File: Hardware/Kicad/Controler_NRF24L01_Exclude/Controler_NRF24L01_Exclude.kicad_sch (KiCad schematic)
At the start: 51 parts, among them J1 Conn_01x02, SW1 SW_Push, SW10 SW_Push, SW11 SW_DIP_x01, SW12 SW_Push, SW13 SW_DIP_x01, SW2 SW_Push, SW3 SW_Push, SW4 SW_Push, SW5 SW_Push, SW6 SW_Push, SW7 SW_Push, SW8 SW_Push, SW9 SW_Push, U1 STM32L412KBTx, U2 MIC5219-3.3YMM, U2 nRF24_Full

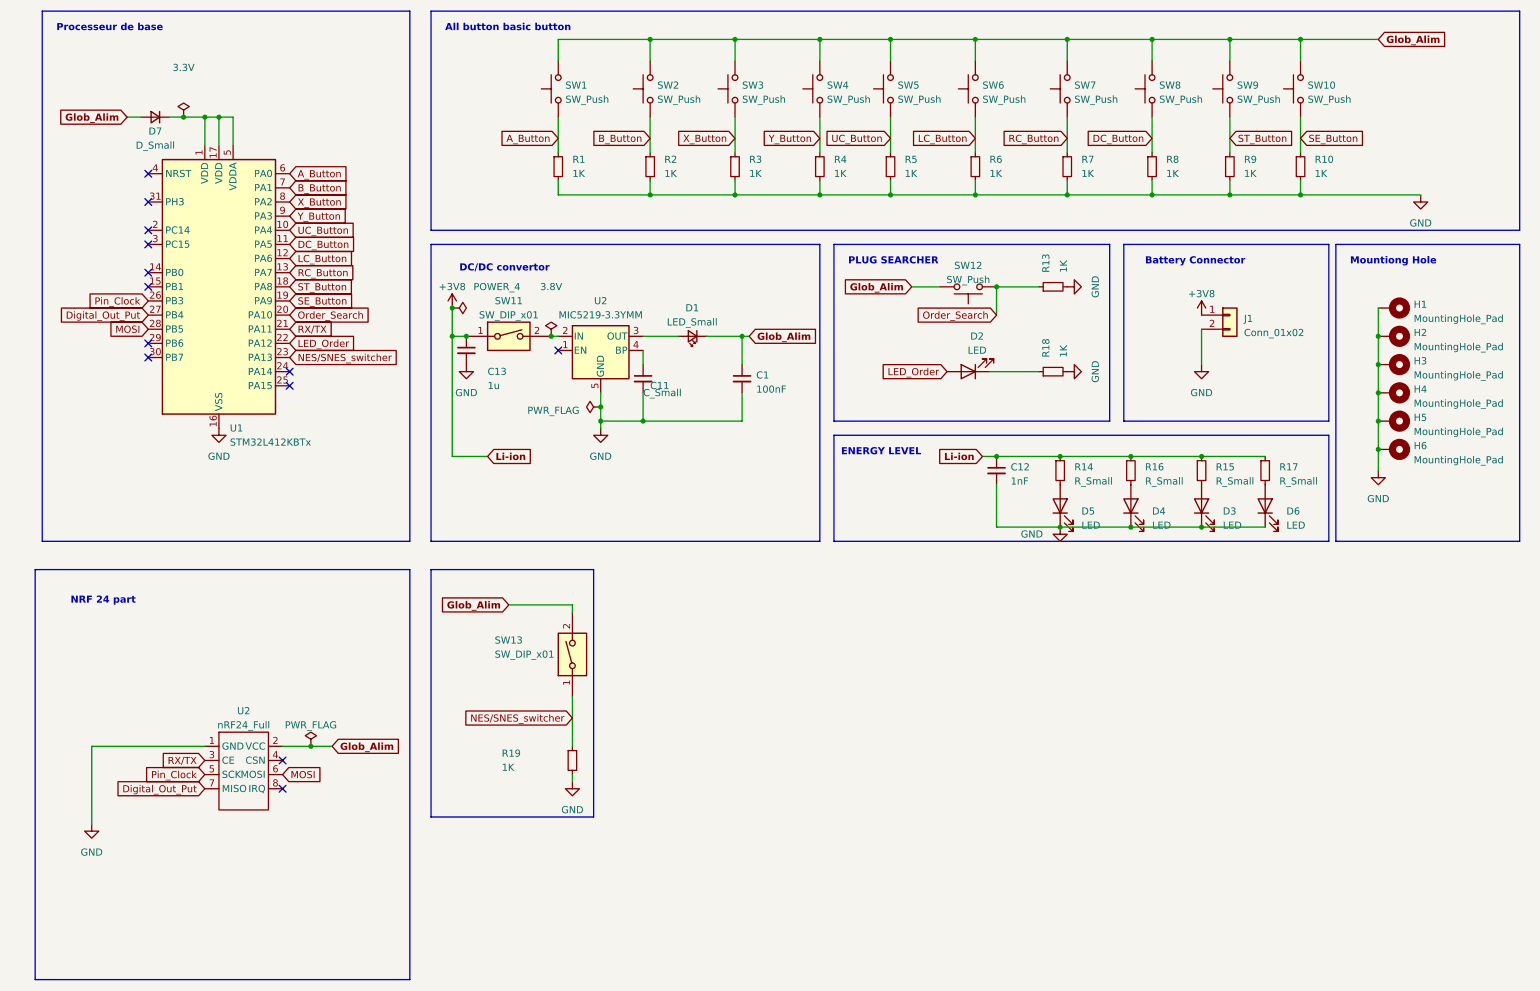
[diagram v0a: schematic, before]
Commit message: correction
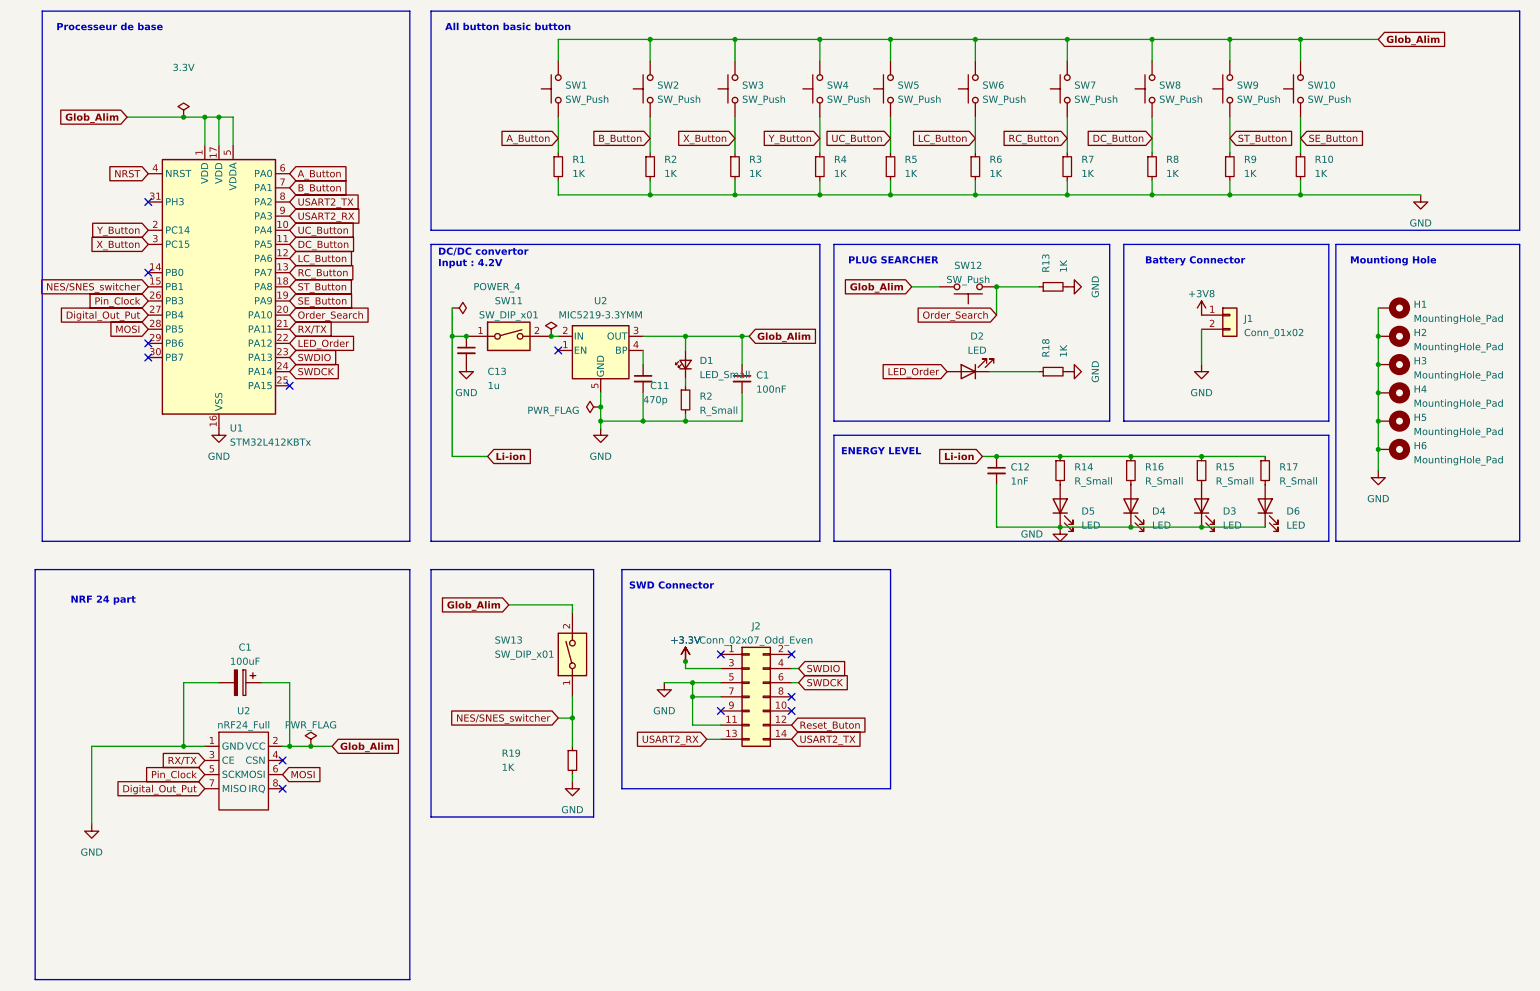
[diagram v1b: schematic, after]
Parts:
- removed D7: D_Small, Diode_SMD:D_0603_1608Metric_Pad1.05x0.95mm_HandSolder, symbol Device:D_Small
- added C1: 100uF, symbol Device:C_Polarized
- added J2: Conn_02x07_Odd_Even, Connector_PinHeader_1.27mm:PinHeader_2x07_P1.27mm_Vertical_SMD, symbol Connector_Generic:Conn_02x07_Odd_Even
- added R2: R_Small, symbol Device:R_Small
- C11: value C_Small -> 470p
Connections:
- net +3V8: no longer C12.1, C13.1, R14.1, R15.1, R16.1, R17.1, SW11.1
- net GND: now also C1.2, J2.11 (Pin_11), J2.5 (Pin_5), J2.7 (Pin_7), R2.2
- net Glob_Alim: now also D1.2 (A), U1.1 (VDD), U1.17 (VDD), U1.5 (VDDA), U2.3 (OUT), C1.1; no longer D1.1 (K)
- net NES/SNES_switcher: now also U1.15 (PB1); no longer U1.23 (PA13)
- net X_Button: now also U1.3 (PC15); no longer U1.8 (PA2)
- net Y_Button: now also U1.2 (PC14); no longer U1.9 (PA3)
- net SWDCK: now reaches U1.24 (PA14)
- net SWDCK: now also J2.6 (Pin_6)
- net NRST: now reaches U1.4 (NRST)
- new net: D1.1 (K), R2.1
- new net +3.3V: J2.3 (Pin_3)
- new net Li-ion: C12.1, C13.1, R14.1, R15.1, R16.1, R17.1, SW11.1
- new net Reset_Buton : J2.12 (Pin_12)
- new net SWDIO: J2.4 (Pin_4), U1.23 (PA13)
- new net USART2_RX: J2.13 (Pin_13), U1.9 (PA3)
- new net USART2_TX: J2.14 (Pin_14), U1.8 (PA2)
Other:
- note added: "DC/DC convertor Input : 4.2V"
- note added: "SWD Connector"
- note removed: "DC/DC convertor"
